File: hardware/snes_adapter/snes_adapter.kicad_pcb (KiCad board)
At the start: 2 copper layers, 96.6 x 25.5 mm, 4 parts, among them J1 CART SLOT TOP ROW, J2 CART SLOT BOTTOM ROW, J3 SNES_Slot

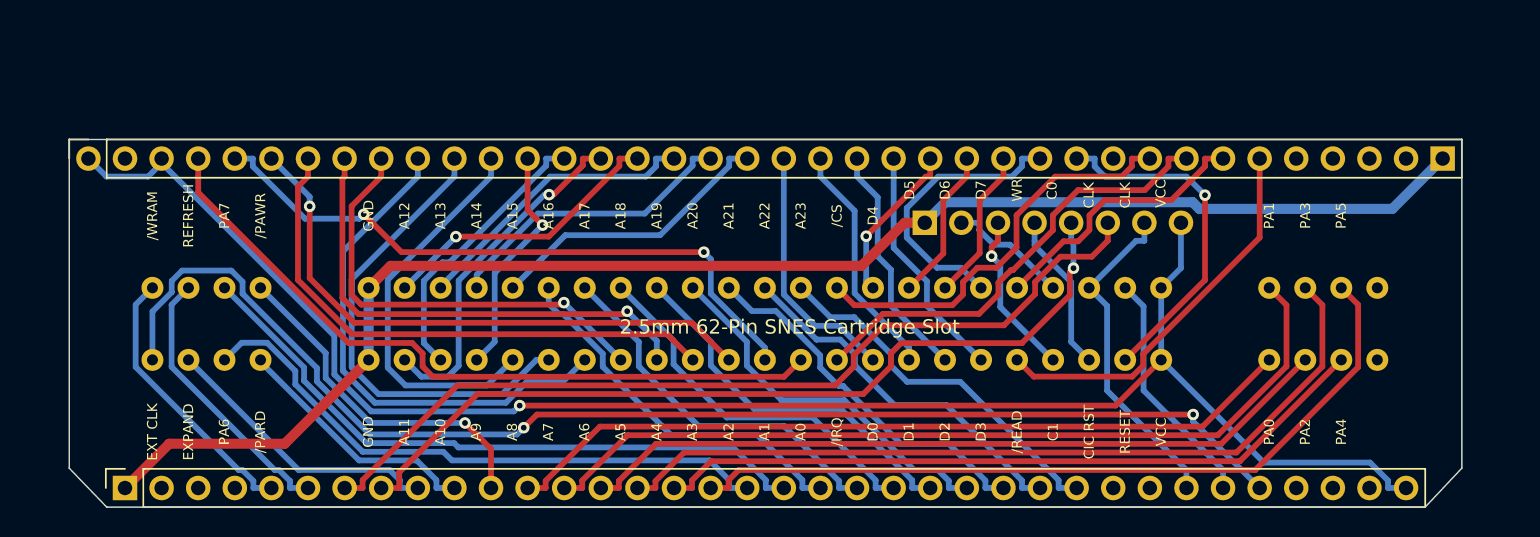
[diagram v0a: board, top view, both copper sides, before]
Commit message: Move SNES updates to clean branch
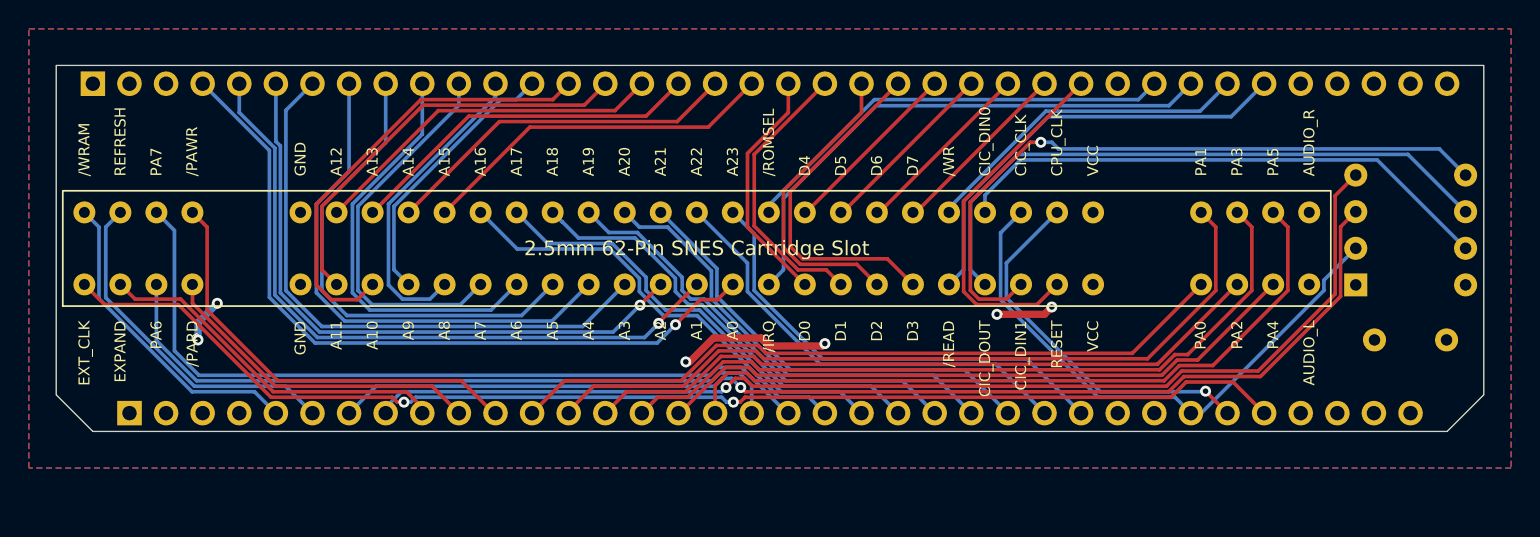
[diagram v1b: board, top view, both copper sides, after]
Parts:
- removed JCIC1: Conn_01x08, Connector_PinHeader_2.54mm:PinHeader_1x08_P2.54mm_Vertical
- added C1: 0.1 uF, Capacitor_THT:C_Disc_D5.0mm_W2.5mm_P5.00mm, B.Cu at (191.8, 94.0)
- added U1: PIC12F629-IP, Package_DIP:DIP-8_W7.62mm, B.Cu at (190.5, 90.2)
- J1: footprint Connector_PinSocket_2.54mm:PinSocket_1x38_P2.54mm_Vertical -> Connector_PinHeader_2.54mm:PinHeader_1x38_P2.54mm_Vertical; moved to B.Cu
- J2: footprint Connector_PinSocket_2.54mm:PinSocket_1x36_P2.54mm_Vertical -> Connector_PinHeader_2.54mm:PinHeader_1x36_P2.54mm_Vertical; moved to B.Cu
- J3: footprint !sanni:SNES Slot -> !OSCR:SNES Slot
- moved J3 38.6 mm to (144.8, 87.6)
- moved J1 5.20 mm to (102.9, 76.2), turned to -90 degrees
- moved J2 5.20 mm to (105.4, 99.1), turned to -90 degrees
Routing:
- net VCC: track 116.9 -> 14.7 mm, vias 1 -> 4
- net GND: track 104.2 -> 3.09 mm, vias 0 -> 2
- net CIC RESET: track 11.1 -> 47.3 mm, vias 0 -> 1
- net CIC DATA 1: track 11.5 -> 43.5 mm, vias 1 -> 0
- net CIC DATA 0: track 8.54 -> 38.1 mm
- net D40: track 59.7 -> 78.8 mm
- net D41: track 62.6 -> 79.2 mm, vias 0 -> 1
- net CLK2: track 23.1 -> 39.7 mm
- net A10: track 19.5 -> 31.3 mm
- net D29: track 45.4 -> 55.0 mm
- net CLK1: track 16.7 -> 26.1 mm, vias 0 -> 1
- net D34: track 16.5 -> 24.0 mm
- net D28: track 41.8 -> 48.9 mm
- net D30: track 19.6 -> 12.8 mm
- net A6: track 35.8 -> 29.1 mm
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- added copper zone on F.Cu, net GND
- added copper zone on B.Cu, net VCC
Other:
- board size 96.6 x 25.5 mm -> 99.1 x 25.4 mm
- board text added: "3v3"
- board text added: "MISO"
- board text added: "MOSI"
- board text added: "SCK"
- board text added: "SS"
- board text removed: "/CS"
- board text removed: "/IRQ"
- board text removed: "/PARD"
- board text removed: "/PAWR"
- board text removed: "/READ"
- board text removed: "/WRAM"
- board text removed: "2.5mm 62-Pin SNES Cartridge Slot"
- board text removed: "A16"
- board text removed: "A17"
- board text removed: "A18"
- board text removed: "A19"
- board text removed: "A20"
- board text removed: "A21"
- board text removed: "A22"
- board text removed: "A23"
- board text removed: "C0"
- board text removed: "C1"
- board text removed: "CIC RST"
- board text removed: "CLK"
- board text removed: "CR"
- board text removed: "EXPAND"
- board text removed: "EXT CLK"
- board text removed: "PA0"
- board text removed: "PA1"
- board text removed: "PA2"
- board text removed: "PA3"
- board text removed: "PA4"
- board text removed: "PA5"
- board text removed: "PA6"
- board text removed: "PA7"
- board text removed: "REFRESH"
- board text removed: "RESET"
- board text removed: "WR"
